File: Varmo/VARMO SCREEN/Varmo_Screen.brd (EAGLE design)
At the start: 160 x 100 mm, 36 parts, among them T2 MMBT2222AL, U1 PCA9670D, U2 LT1813CS8, U3 90814-0210

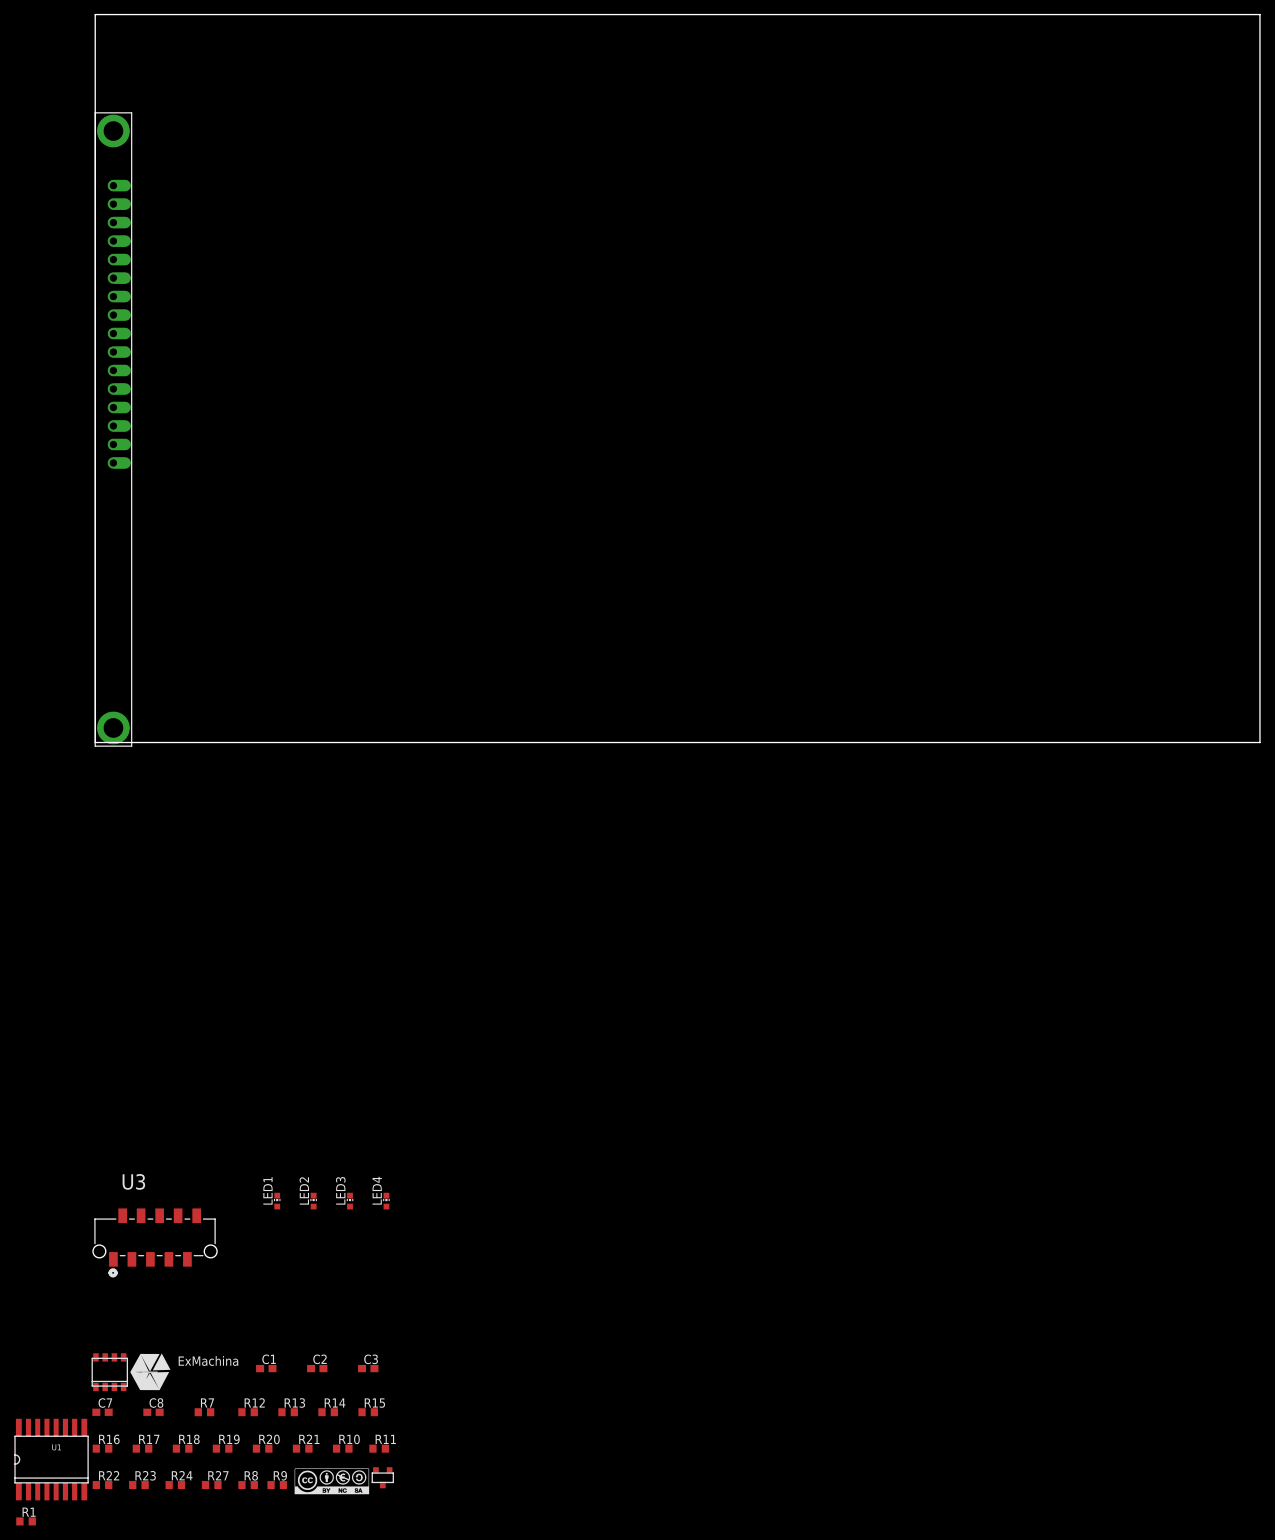
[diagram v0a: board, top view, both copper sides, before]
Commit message: Re routing the board
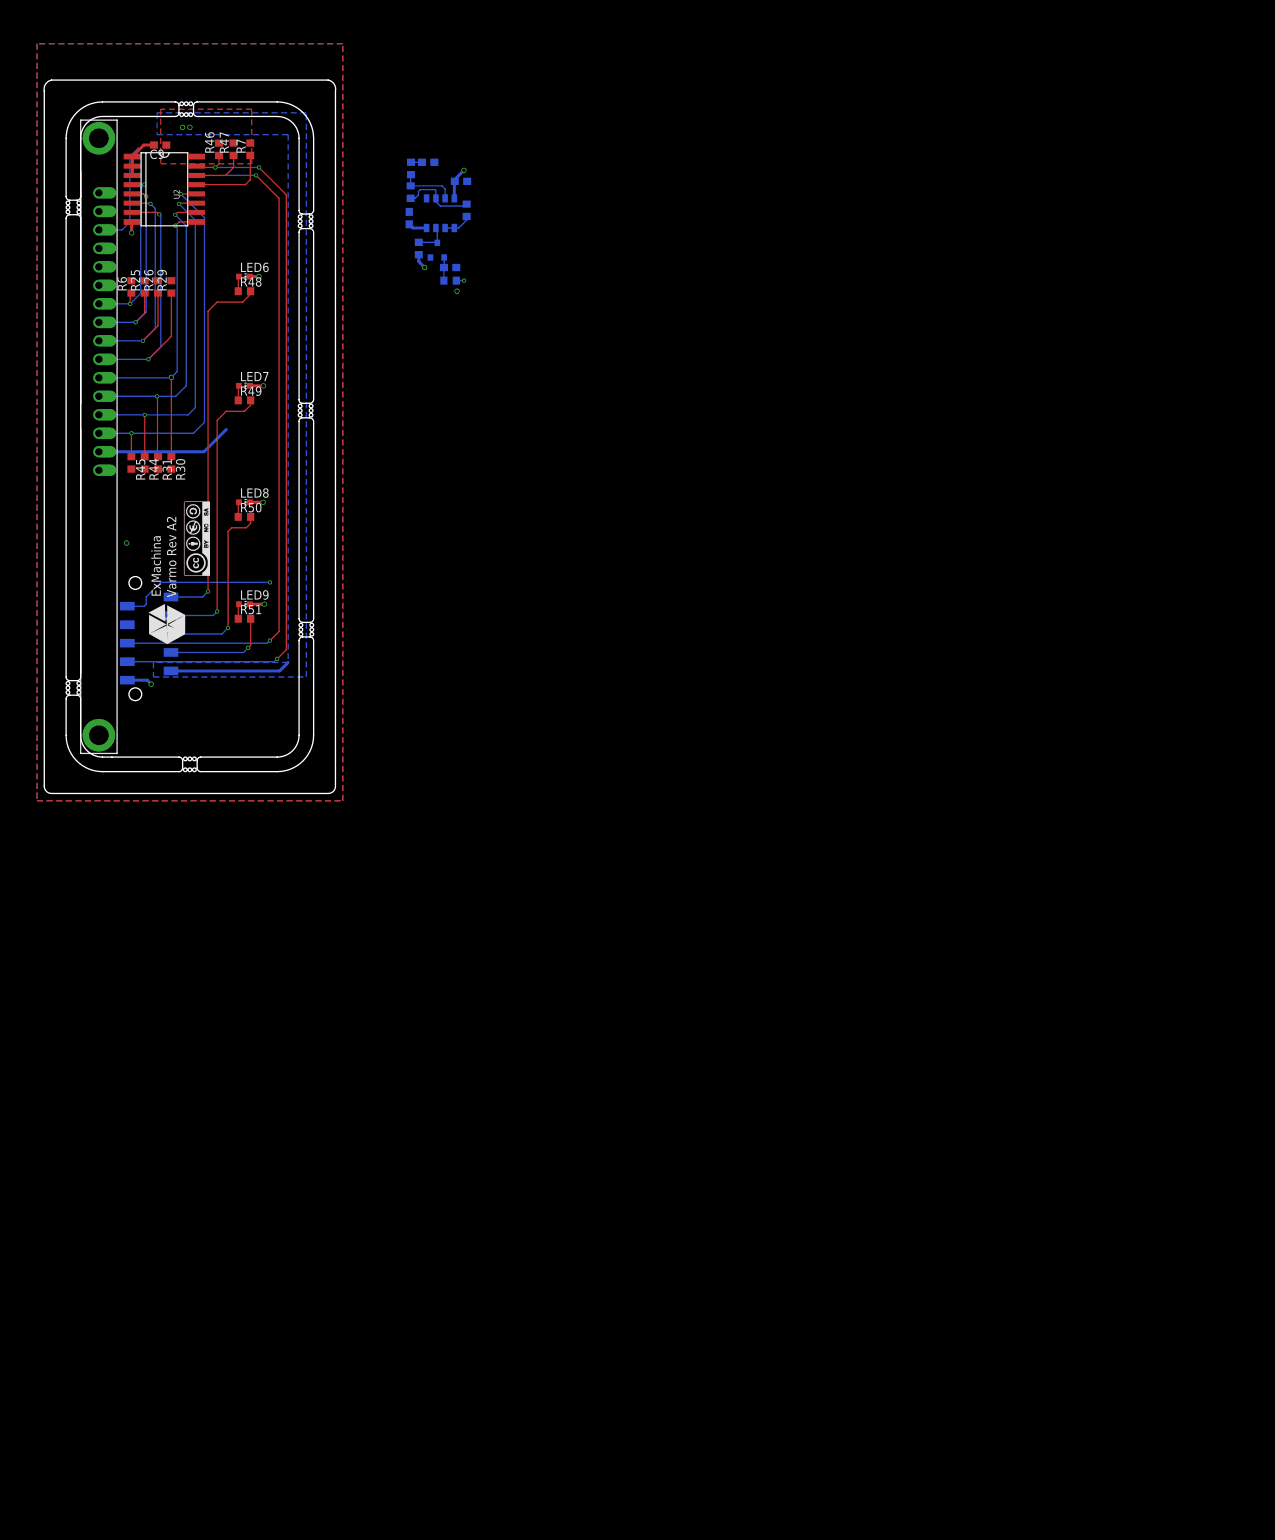
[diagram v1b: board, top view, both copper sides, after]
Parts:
- removed C1, C3, C7, C8: 0.1uF, rcl:C0603
- removed C2: 4.7uF, rcl:C0603
- removed LCD2: MC41605A12W, midas:CONNECTOR
- removed LED1, LED2, LED3, LED4: Blue, led:CHIP-LED0603
- removed R10, R22, R23, R24, R27, R8, R9: 1k, rcl:R0603
- removed R11: 10k, rcl:R0603
- removed R12, R13, R14, R15, R16, R17, R18, R19, R20, R21: 4.7k, rcl:R0603
- removed T2: MMBT2222AL, transistor:SOT−23
- removed U$1: CC-BY-NC-SA, cc-by-sa:CC-BY-NC-SA
- removed U$2: EXMACHINA-LOGO-NAME, exmachina:EXM-LOGO-BASELINE
- removed U3: 90814-0210, Molex_By_element14_Batch_1:MOLEX_90814-0210
- added C10, C4, C6, C9: 0.1uF, rcl:C0603
- added C5: 4.7uF, rcl:C0603
- added LCD1: MC41605A12W, midas:CONNECTOR
- added LED6, LED7, LED8, LED9: Blue, led:CHIP-LED0603
- added R2, R3, R4, R48, R49, R50, R51: 1k, rcl:R0603
- added R25, R26, R29, R30, R31, R44, R45, R46, R47, R6: 4.7k, rcl:R0603
- added R5: 10k, rcl:R0603
- added T1: MMBT2222AL, transistor:SOT−23
- added U$5: CC-BY-NC-SA, cc-by-sa:CC-BY-NC-SA
- added U$7: EXMACHINA-LOGO-NAME, exmachina:EXM-LOGO-BASELINE
- added U5: 90814-0210, Molex_By_element14_Batch_1:MOLEX_90814-0210
- R1: value 4.7k -> 100R
- R7: value 100R -> 4.7k
- U1: value PCA9670D -> LT1813CS8; device NXP:SOT162-1 -> lineartechnology:SOIC8
- U2: value LT1813CS8 -> PCA9670D; device lineartechnology:SOIC8 -> NXP:SOT162-1
- moved R1 180.1 mm to (48.8, 63.5), flipped to the bottom
- moved U1 179.4 mm to (47.4, 72.7), flipped to the bottom
- moved R7 173.6 mm to (21.3, 81.5), turned to 90 degrees
- moved U2 162.7 mm to (9.50, 76.0), turned to 270 degrees
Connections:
- removed net N$10: LED1.A, R22.1
- removed net N$11: LED2.A, R23.1
- removed net N$12: LED3.A, R24.1
- removed net N$13: LED4.A, R27.1
- removed net N$6: R8.1, T2.3, U2.3
- removed net N$7: R9.2, U2.1, U2.2
- removed net N$8: R10.2, R9.1, U2.6
- removed net N$9: R10.1, R11.2, U2.7
- removed net RESET: R1.1, U1.13
- new net N$14: R3.1, R4.2, U1.6
- new net N$17: R4.1, R5.2, U1.7
- new net N$2: C4.1, R1.2, T1.1
- new net N$22: LED7.A, R49.1
- new net N$24: LED8.A, R50.1
- new net N$29: LED9.A, R51.1
- new net N$3: R2.1, T1.3, U1.3
- new net N$4: LED6.A, R48.1
- new net N$5: R3.2, U1.1, U1.2
- net +3V3: now also C9.1, R46.2, R47.2, R7.2, U2.16, U5.2; no longer C8.1, R1.2, R20.2, R21.2, U1.16, U3.2
- net +5V/1: now also C6.1, LCD1.2, LCD1.4, LCD1.6, R2.2, R25.2, R26.2, R29.2, R30.2, R31.2, R44.2, R45.2, R6.2, U1.8, U5.1; no longer C3.1, LCD2.2, LCD2.4, LCD2.6, R12.2, R13.2, R14.2, R15.2, R16.2, R17.2, R18.2, R19.2, R8.2, U2.8, U3.1
- net D0: now also LCD1.7, R6.1, U2.4; no longer LCD2.7, R12.1, U1.4
- net D1: now also LCD1.8, R25.1, U2.5; no longer LCD2.8, R13.1, U1.5
- net D2: now also LCD1.9, R26.1, U2.6; no longer LCD2.9, R14.1, U1.6
- net D3: now also LCD1.10, R29.1, U2.7; no longer LCD2.10, R15.1, U1.7
- net D4: now also LCD1.11, R30.1, U2.9; no longer LCD2.11, R16.1, U1.9
- net D5: now also LCD1.12, R31.1, U2.10; no longer LCD2.12, R17.1, U1.10
- net D6: now also LCD1.13, R44.1, U2.11; no longer LCD2.13, R18.1, U1.11
- net D7: now also LCD1.14, R45.1, U2.12; no longer LCD2.14, R19.1, U1.12
- net GND1: now also C10.2, C4.2, C5.2, C6.2, C9.2, LCD1.1, LCD1.16, LCD1.5, LED6.C, LED7.C, LED8.C, LED9.C, T1.2, U1.5, U2.1, U2.2, U2.3, U2.8, U5.7; no longer C1.2, C2.2, C3.2, C7.2, C8.2, LCD2.1, LCD2.16, LCD2.5, LED1.C, LED2.C, LED3.C, LED4.C, T2.2, U1.1, U1.2, U1.8, U2.5, U3.7
- net LED_STATUS_1: now also R48.2, U5.10; no longer R22.2, U3.10
- net LED_STATUS_2: now also R49.2, U5.8; no longer R23.2, U3.8
- net LED_STATUS_3: now also R50.2, U5.6; no longer R24.2, U3.6
- net LED_STATUS_4: now also R51.2, U5.4; no longer R27.2, U3.4
- net N$1: now also R7.1, U2.13; no longer C1.1, R7.2, T2.1
- net PWM_CONTRASTE: now also R1.1, U5.9; no longer R7.1, U3.9
- net SCL: now also R47.1, U2.14, U5.5; no longer R21.1, U1.14, U3.5
- net SDA: now also R46.1, U2.15, U5.3; no longer R20.1, U1.15, U3.3
- net VEE: now also C10.1, LCD1.15, U1.4; no longer C7.1, LCD2.15, U2.4
- net VO: now also C5.1, LCD1.3, R5.1; no longer C2.1, LCD2.3, R11.1
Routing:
- net SDA: track 0.00 -> 100.9 mm, vias 0 -> 3
- net SCL: track 0.00 -> 96.9 mm, vias 0 -> 2
- net D7: track 0.00 -> 53.2 mm, vias 0 -> 2
- net LED_STATUS_1: track 0.00 -> 51.1 mm, vias 0 -> 1
- net D6: track 0.00 -> 50.8 mm, vias 0 -> 2
- net D5: track 0.00 -> 48.1 mm, vias 0 -> 2
- net D4: track 0.00 -> 45.3 mm, vias 0 -> 2
- net D3: track 0.00 -> 41.7 mm, vias 0 -> 2
- net LED_STATUS_2: track 0.00 -> 38.9 mm, vias 0 -> 1
- net D2: track 0.00 -> 35.8 mm, vias 0 -> 2
- net D1: track 0.00 -> 29.5 mm, vias 0 -> 2
- net LED_STATUS_3: track 0.00 -> 25.9 mm, vias 0 -> 1
- net D0: track 0.00 -> 24.7 mm, vias 0 -> 2
- net PWM_CONTRASTE: track 0.00 -> 22.8 mm, vias 0 -> 2
- net VEE: track 0.00 -> 21.4 mm
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- added copper zone on layer 1, net +3V3
- added copper zone on layer 16, net +3V3
- added copper zone on layer 1, net +5V/1
- added copper zone on layer 16, net GND1
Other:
- board size 160 x 100 mm -> 40 x 98 mm
- board text added: "Varmo Rev A2"
